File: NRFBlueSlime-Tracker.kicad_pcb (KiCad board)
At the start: 4 copper layers, 21.3 x 30.7 mm, 48 parts, among them J1 532610271, J3 USB_C_Receptacle_USB2.0_16P, Q1 AO3401A, SW1 TS-1088-AR02016, SW2 SK-3296S-01-L1, U1 MDBT50Q-1MV2, U2 ICM-42688-P, U3 LIS2MDL, U4 ME6211C33R5G, U5 TP4057-42-SOT26-R, X1 S2D32.768KB20F30T

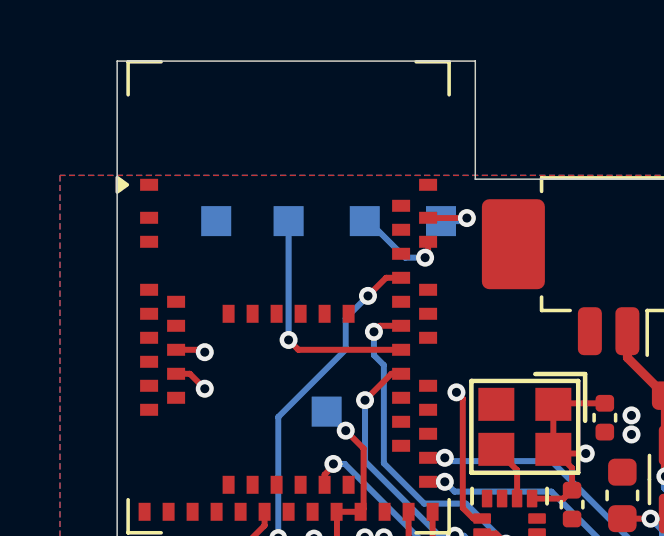
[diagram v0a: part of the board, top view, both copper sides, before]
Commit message: fix gnd testpad
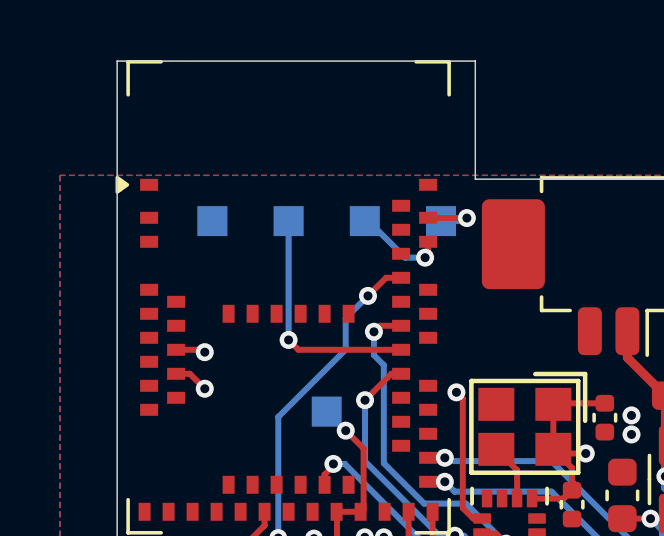
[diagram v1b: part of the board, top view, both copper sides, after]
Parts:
- moved TP5 0.13 mm to (73.7, 27.9)
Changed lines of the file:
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@@
 	(footprint "TestPoint:TestPoint_Pad_1.0x1.0mm"
 		(layer "B.Cu")
-		(at 73.787 27.94 180)
+		(at 73.66 27.94 180)
 		(descr "SMD rectangular pad as test Point, square 1.0mm side length")
 		(tags "test point SMD pad rectangle square")

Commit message: use copper fill in in1cu layer
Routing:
- added copper zone on In1.Cu, net GND
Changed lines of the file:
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@@
 		(net 2)
 		(net_name "GND")
-		(layers "F&B.Cu")
+		(layers "F.Cu" "In1.Cu" "B.Cu")
 		(hatch edge 0.5)
 		(connect_pads
